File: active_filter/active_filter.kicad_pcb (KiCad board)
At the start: 2 copper layers, 26.4 x 22.9 mm, 15 parts, among them J0 Conn_01x03_MountingPin, J1 Conn_01x03_MountingPin, U1 ADA4062-2

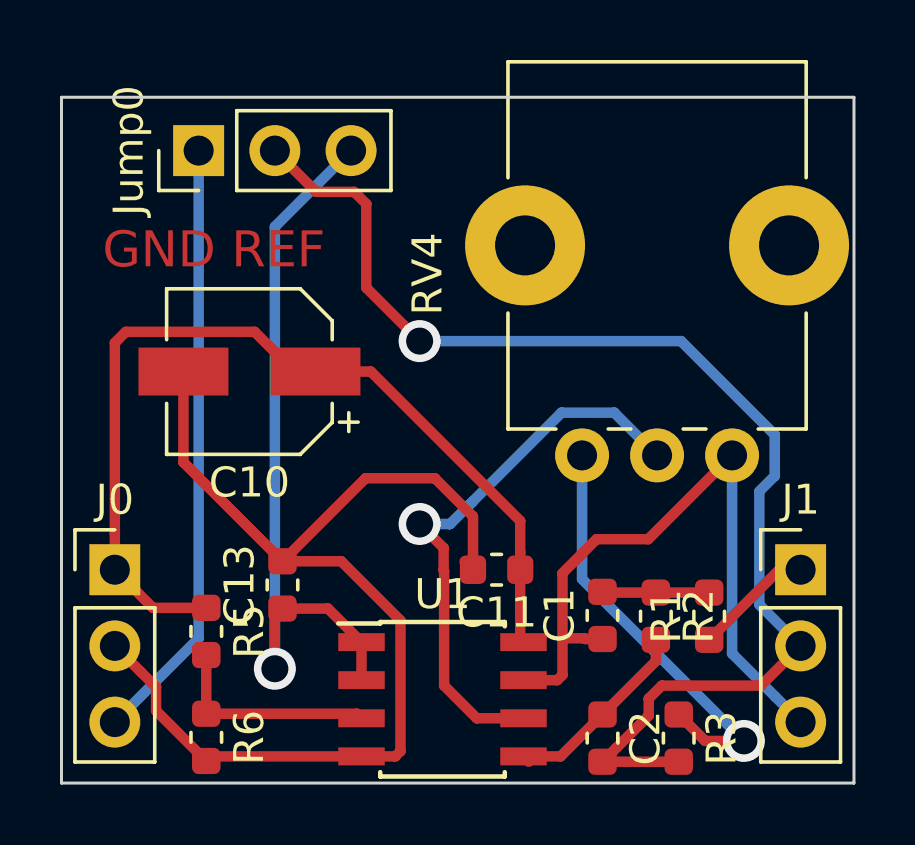
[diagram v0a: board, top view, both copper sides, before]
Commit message: updated pcb and bom
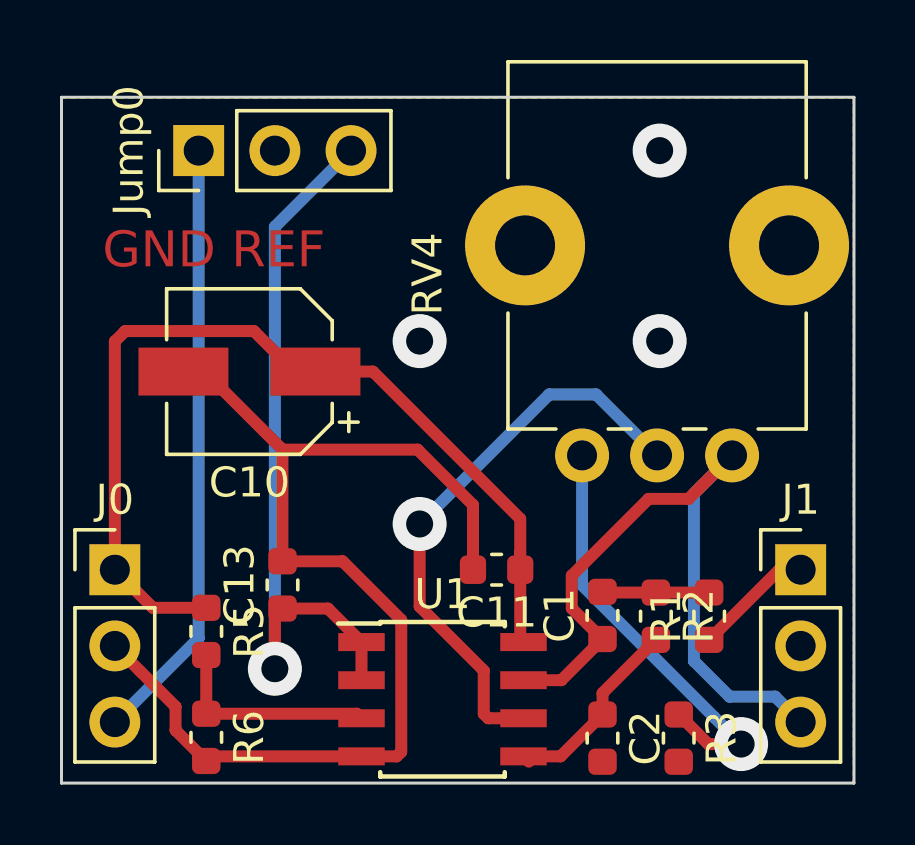
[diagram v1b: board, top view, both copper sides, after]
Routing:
- net COM: track 41.1 -> 0.00 mm, vias 1 -> 3
- net OUT: track 23.2 -> 24.5 mm
- added copper zone on B.Cu, net COM
- added copper zone on F.Cu, net COM
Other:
- net class Default: trace_width 0.35 -> 0.4; via_dia 1.4 -> 1.8
- rule via_min_size: 1.905 -> 1.8
